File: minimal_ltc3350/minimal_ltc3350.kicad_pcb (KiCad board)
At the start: 4 copper layers, 64.8 x 49.5 mm, 90 parts, among them J1 CLP-102-02-G-D-BE, J2 CLP-102-02-G-D-BE, J3 CLP-102-02-G-D-BE, J4 CLP-102-02-G-D-BE, J5 CLP-102-02-G-D-BE, Q1 20.0 V, Q2 20.0 V, Q3 20 V, Q4 20 V, Q5 20.0 V, Q6 8 V, Q7 8 V, Q8 8 V, Q9 8 V, U1 LTC3350EUHF-PBF

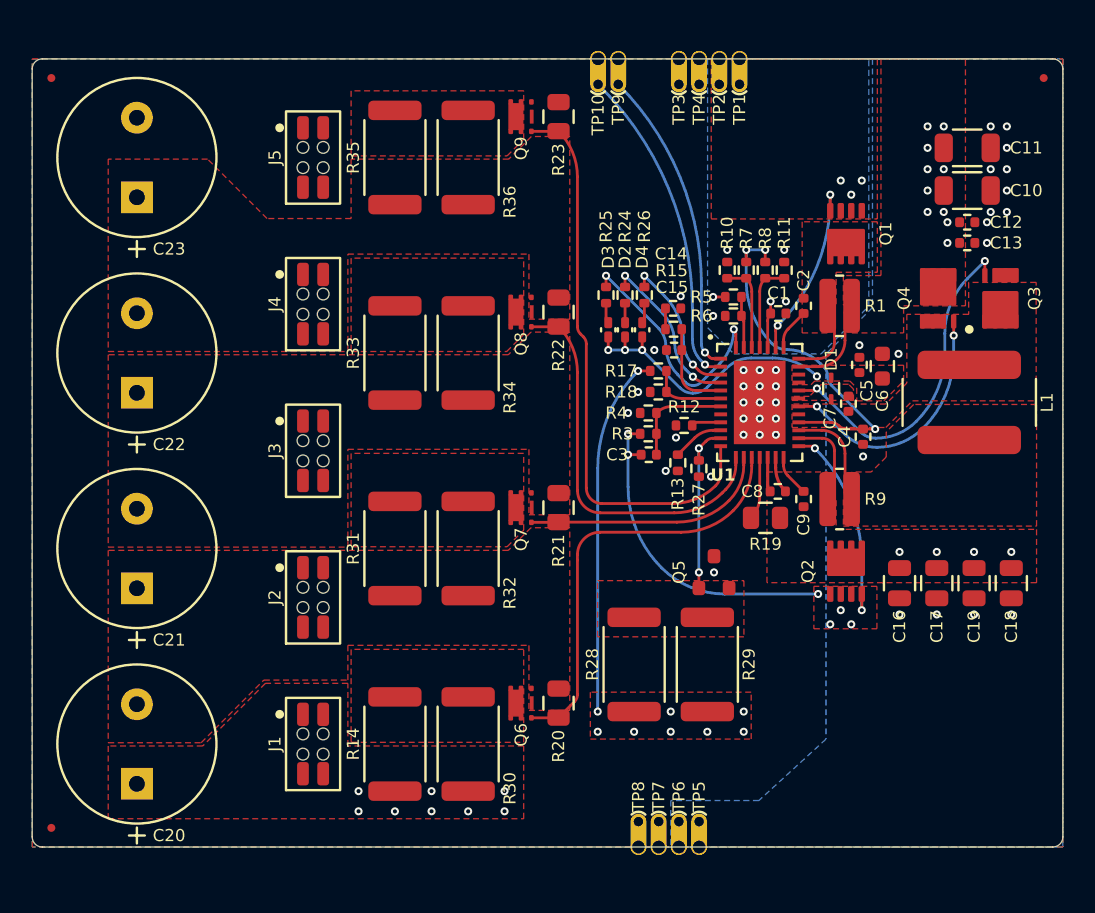
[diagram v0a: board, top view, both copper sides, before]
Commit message: Update KiCad project files: PCB layout, project settings, and schematic
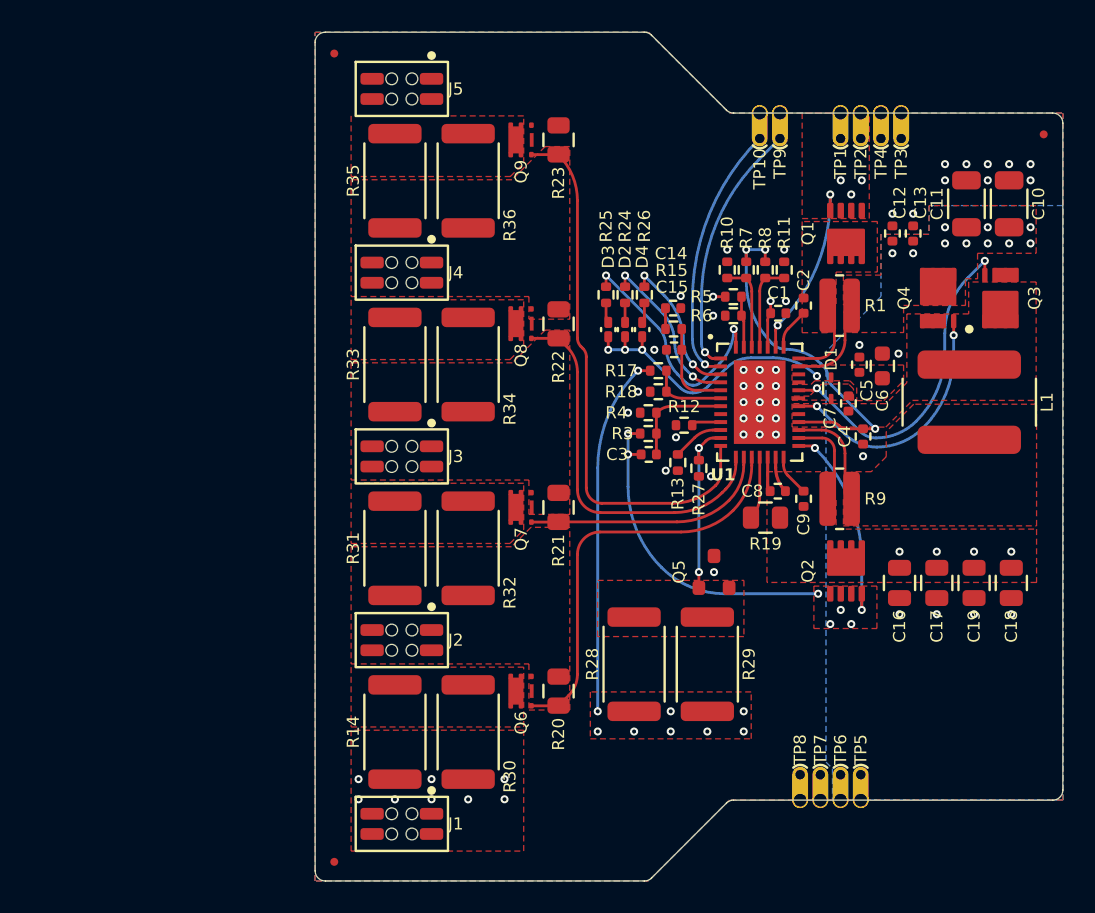
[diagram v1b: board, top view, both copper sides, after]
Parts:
- removed C20, C21, C22, C23: 10 F, capacitor_footprints:C_197x394_H31_5_5_0x10Metric
- moved FID1 17.9 mm to (113.0, 117.8)
- moved FID2 17.8 mm to (113.0, 67.0)
- moved TP3 14.4 mm to (148.6, 70.7)
- moved TP4 11.9 mm to (147.3, 70.7)
- moved TP10 10.7 mm to (139.7, 70.7)
- moved TP9 10.7 mm to (141.0, 70.7)
- moved TP5 10.6 mm to (146.1, 113.9)
- moved TP6 10.6 mm to (144.8, 113.9)
- moved TP7 10.6 mm to (143.5, 113.9)
- moved TP8 10.6 mm to (142.2, 113.9)
- moved TP2 9.52 mm to (146.1, 70.7)
- moved J1 7.50 mm to (117.2, 115.4), turned to -90 degrees
- moved TP1 7.20 mm to (144.8, 70.7)
- moved J5 7.05 mm to (117.2, 69.2), turned to -90 degrees
- moved J2 6.19 mm to (117.2, 103.8), turned to -90 degrees
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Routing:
- net /SDA: track 20.4 -> 16.5 mm
- net /SCL: track 19.4 -> 16.1 mm
- net /CAPRTN: track 36.1 -> 34.6 mm
- net /CAP3: track 26.9 -> 26.1 mm
- net /CAP1: track 24.9 -> 24.3 mm
- removed copper zone on B.Cu, net /VIN
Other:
- board size 64.8 x 49.5 mm -> 47 x 53.3 mm
